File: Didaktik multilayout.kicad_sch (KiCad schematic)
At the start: 103 parts, among them J1 Conn_01x04_MountingPin, J2 AVR-ISP-6, SW1 SW_Push_45deg, SW10 SW_Push_45deg, SW11 SW_Push_45deg, SW12 SW_Push_45deg, SW13 SW_Push_45deg, SW14 SW_Push_45deg, SW15 SW_Push_45deg, SW16 SW_Push_45deg, SW17 SW_Push_45deg, SW18 SW_Push_45deg, SW19 SW_Push_45deg, SW2 SW_Push_45deg, SW20 SW_Push_45deg, SW21 SW_Push_45deg, SW22 SW_Push_45deg, SW23 SW_Push_45deg, SW24 SW_Push_45deg, SW25 SW_Push_45deg, SW26 SW_Push_45deg, SW27 SW_Push_45deg, SW28 SW_Push_45deg, SW29 SW_Push_45deg, SW3 SW_Push_45deg, SW30 SW_Push_45deg, SW31 SW_Push_45deg, SW32 SW_Push_45deg, SW33 SW_Push_45deg, SW34 SW_Push_45deg, SW35 SW_Push_45deg, SW36 SW_Push_45deg, SW37 SW_Push_45deg, SW38 SW_Push_45deg, SW39 SW_Push_45deg, SW4 SW_Push_45deg, SW40 SW_Push_45deg, SW5 SW_Push_45deg, SW6 SW_Push_45deg, SW7 SW_Push_45deg, SW8 SW_Push_45deg, SW9 SW_Push_45deg, U1 ATmega32U4-M, Y1 Crystal_GND24_Small

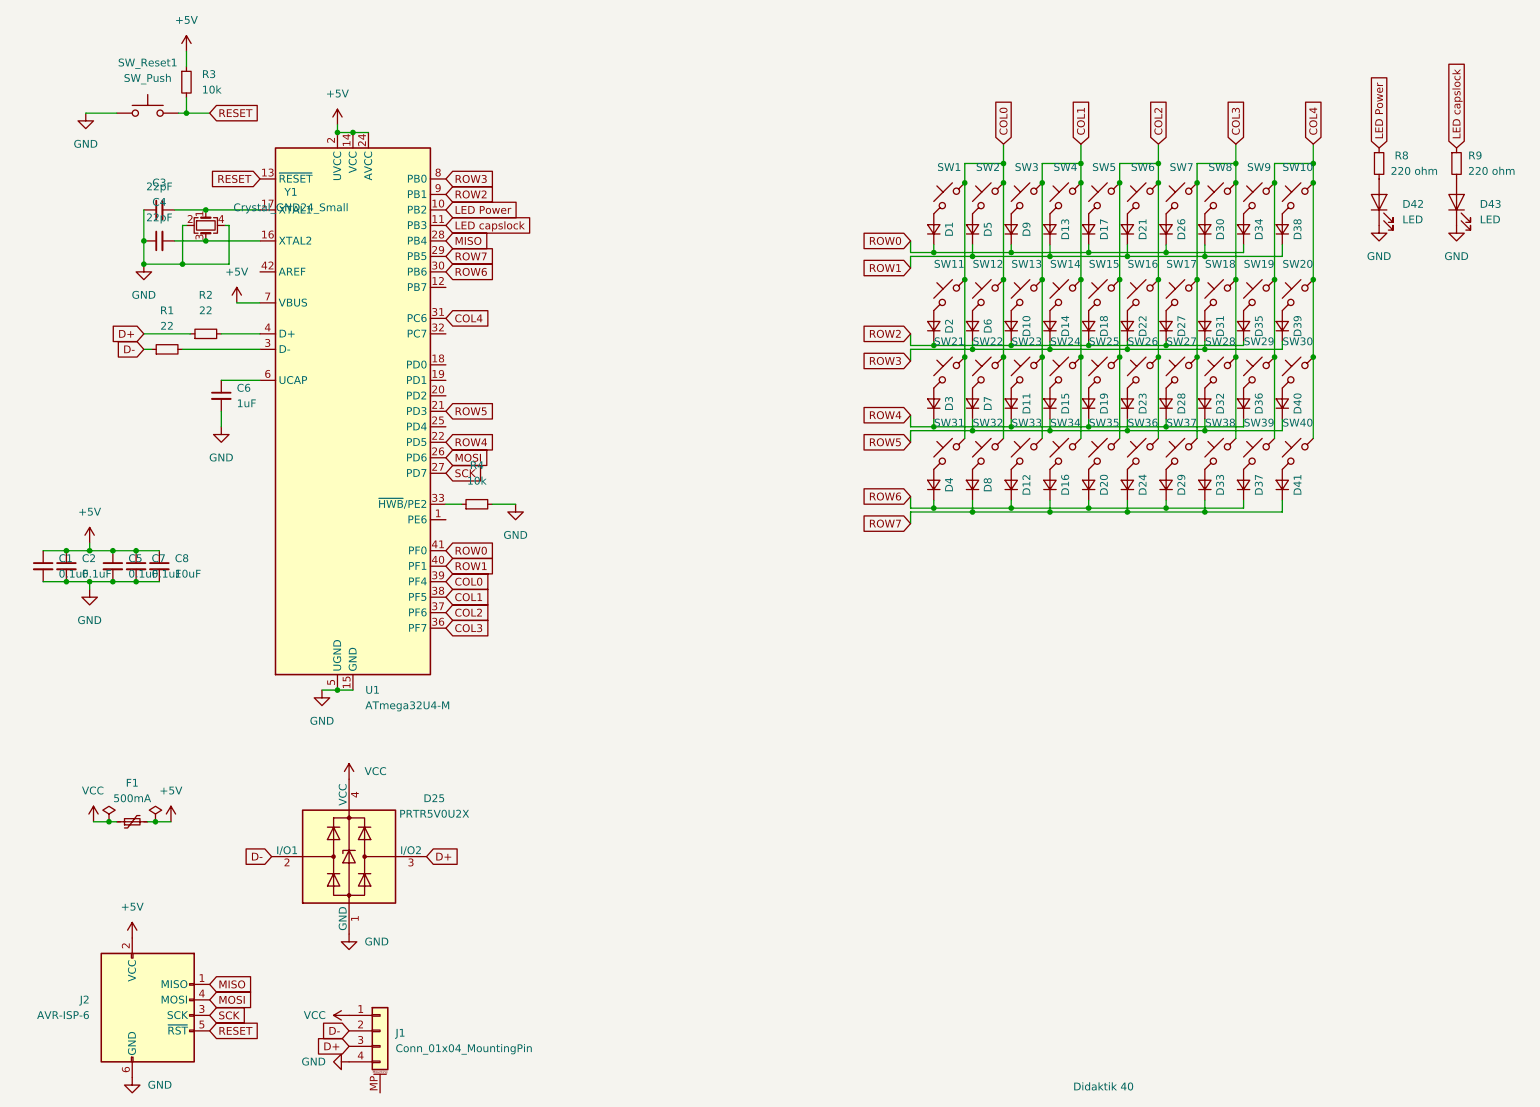
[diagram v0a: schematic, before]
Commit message: routing multipcb
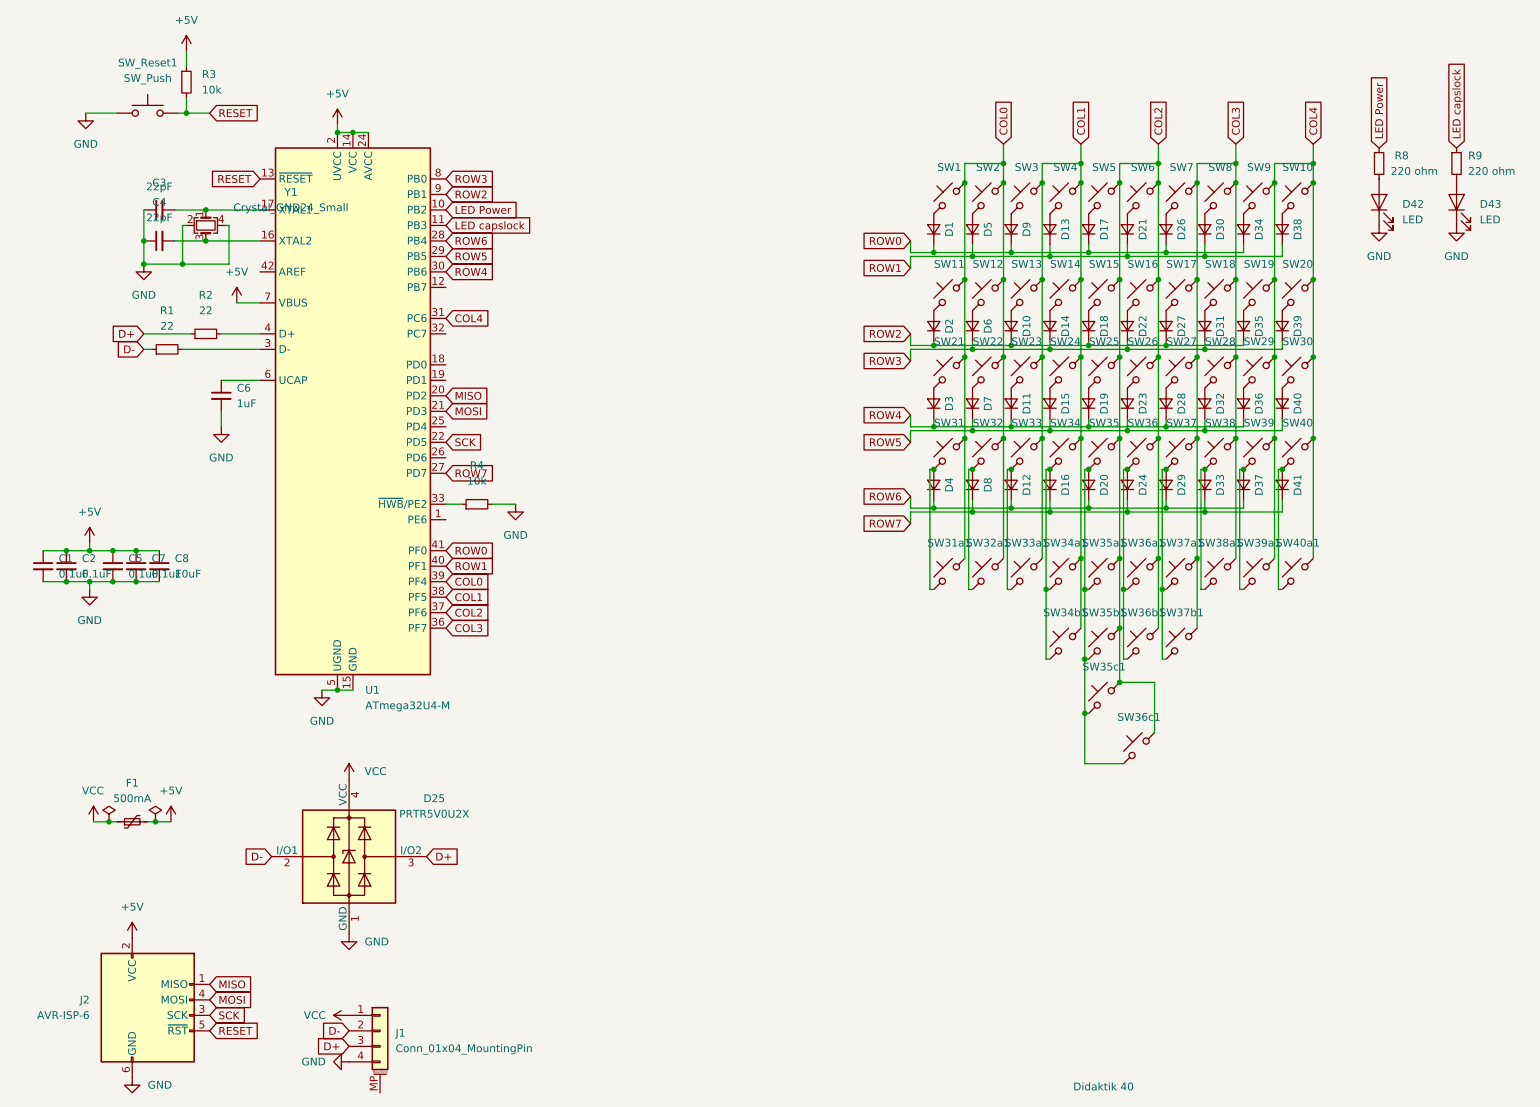
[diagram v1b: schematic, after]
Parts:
- added SW31a1, SW32a1, SW33a1, SW34a1, SW37a1, SW38a1, SW39a1, SW40a1: SW_Push_45deg, Keebio-Parts:MX-Alps-Choc-1U-NoLED, symbol Switch:SW_Push_45deg
- added SW34b1, SW37b1: SW_Push_45deg, Keebio-Parts:MX-Alps-Choc-3U-NoLED-StabFlip, symbol Switch:SW_Push_45deg
- added SW35a1, SW36a1: SW_Push_45deg, Keebio-Parts:MX-Alps-Choc-1.5U-NoLED, symbol Switch:SW_Push_45deg
- added SW35b1, SW36b1: SW_Push_45deg, Keebio-Parts:MX-Alps-Choc-2U-NoLED-StabFlip, symbol Switch:SW_Push_45deg
- added SW35c1: SW_Push_45deg, Keebio-Parts:MX-Alps-Choc-6U-NoLED-StabFlip, symbol Switch:SW_Push_45deg
- added SW36c1: SW_Push_45deg, Keebio-Parts:MX-Alps-Choc-7U-NoLED-StabFlip, symbol Switch:SW_Push_45deg
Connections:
- net COL0: now also SW31a1.1, SW32a1.1
- net COL1: now also SW33a1.1, SW34a1.1, SW34b1.1
- net COL2: now also SW35a1.1, SW35b1.1, SW35c1.1, SW36a1.1, SW36b1.1, SW36c1.1
- net COL3: now also SW37a1.1, SW37b1.1, SW38a1.1
- net COL4: now also SW39a1.1, SW40a1.1
- net MISO: now also U1.20 (PD2); no longer U1.28 (PB4)
- net MOSI: now also U1.21 (PD3); no longer U1.26 (PD6)
- net ROW4: now also U1.30 (PB6); no longer U1.22 (PD5)
- net ROW5: now also U1.29 (PB5); no longer U1.21 (PD3)
- net ROW6: now also U1.28 (PB4); no longer U1.30 (PB6)
- net ROW7: now also U1.27 (PD7); no longer U1.29 (PB5)
- net SCK: now also U1.22 (PD5); no longer U1.27 (PD7)
- net at D37.2 (A), SW39.2: now also SW39a1.2
- net at D8.2 (A), SW32.2: now also SW32a1.2
- net at D33.2 (A), SW38.2: now also SW38a1.2
- net at D20.2 (A), SW35.2: now also SW35a1.2, SW35b1.2, SW35c1.2, SW36c1.2
- net at D41.2 (A), SW40.2: now also SW40a1.2
- net at D24.2 (A), SW36.2: now also SW36a1.2, SW36b1.2
- net at D12.2 (A), SW33.2: now also SW33a1.2
- net at D16.2 (A), SW34.2: now also SW34a1.2, SW34b1.2
- net at D29.2 (A), SW37.2: now also SW37a1.2, SW37b1.2
- net at D4.2 (A), SW31.2: now also SW31a1.2

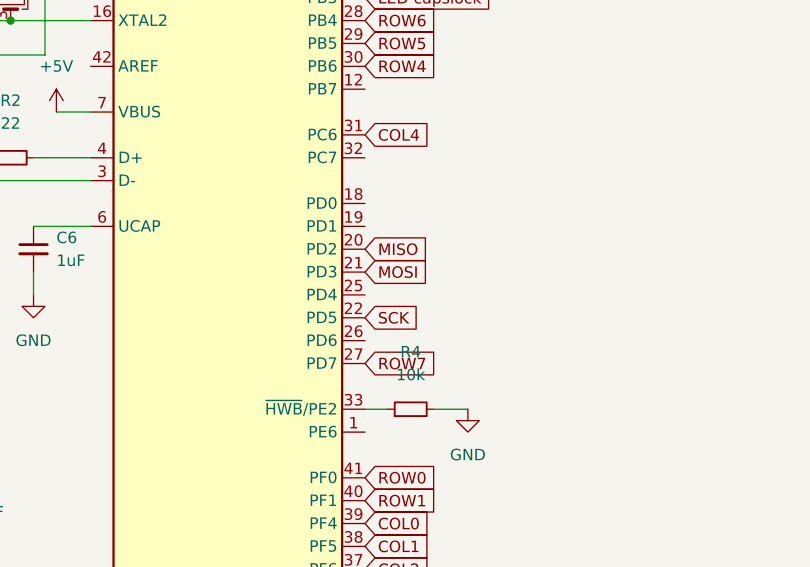
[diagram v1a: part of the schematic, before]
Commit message: set up multilayout
need to check if all switches are really routed
maybe get rid of 2U
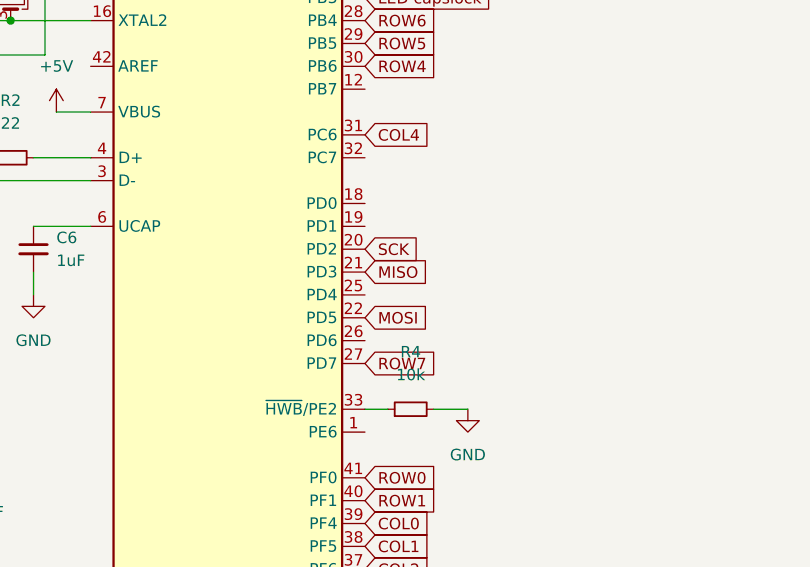
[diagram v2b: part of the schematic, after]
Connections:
- net MISO: now also U1.21 (PD3); no longer U1.20 (PD2)
- net MOSI: now also U1.22 (PD5); no longer U1.21 (PD3)
- net SCK: now also U1.20 (PD2); no longer U1.22 (PD5)
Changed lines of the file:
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@@
     )
   )
-  (global_label "MOSI" (shape input) (at 85.09 78.74 0) (fields_autoplaced)
+  (global_label "MOSI" (shape input) (at 85.09 83.82 0) (fields_autoplaced)
     (effects (font (size 1.27 1.27)) (justify left))
-    (property "Intersheet References" "${INTERSHEET_REFS}" (id 0) (at 92.0993 78.6606 0)
+    (property "Intersheet References" "${INTERSHEET_REFS}" (id 0) (at 92.0993 83.7406 0)
       (effects (font (size 1.27 1.27)) (justify left) hide)
     )
@@
     )
   )
-  (global_label "MISO" (shape input) (at 85.09 76.2 0) (fields_autoplaced)
+  (global_label "MISO" (shape input) (at 85.09 78.74 0) (fields_autoplaced)
     (effects (font (size 1.27 1.27)) (justify left))
-    (property "Intersheet References" "${INTERSHEET_REFS}" (id 0) (at 92.0993 76.1206 0)
+    (property "Intersheet References" "${INTERSHEET_REFS}" (id 0) (at 92.0993 78.6606 0)
       (effects (font (size 1.27 1.27)) (justify left) hide)
     )
@@
     )
   )
-  (global_label "SCK" (shape input) (at 85.09 83.82 0) (fields_autoplaced)
+  (global_label "SCK" (shape input) (at 85.09 76.2 0) (fields_autoplaced)
     (effects (font (size 1.27 1.27)) (justify left))
-    (property "Intersheet References" "${INTERSHEET_REFS}" (id 0) (at 91.2526 83.7406 0)
+    (property "Intersheet References" "${INTERSHEET_REFS}" (id 0) (at 91.2526 76.1206 0)
       (effects (font (size 1.27 1.27)) (justify left) hide)
     )
